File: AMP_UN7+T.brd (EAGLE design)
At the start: 31 parts

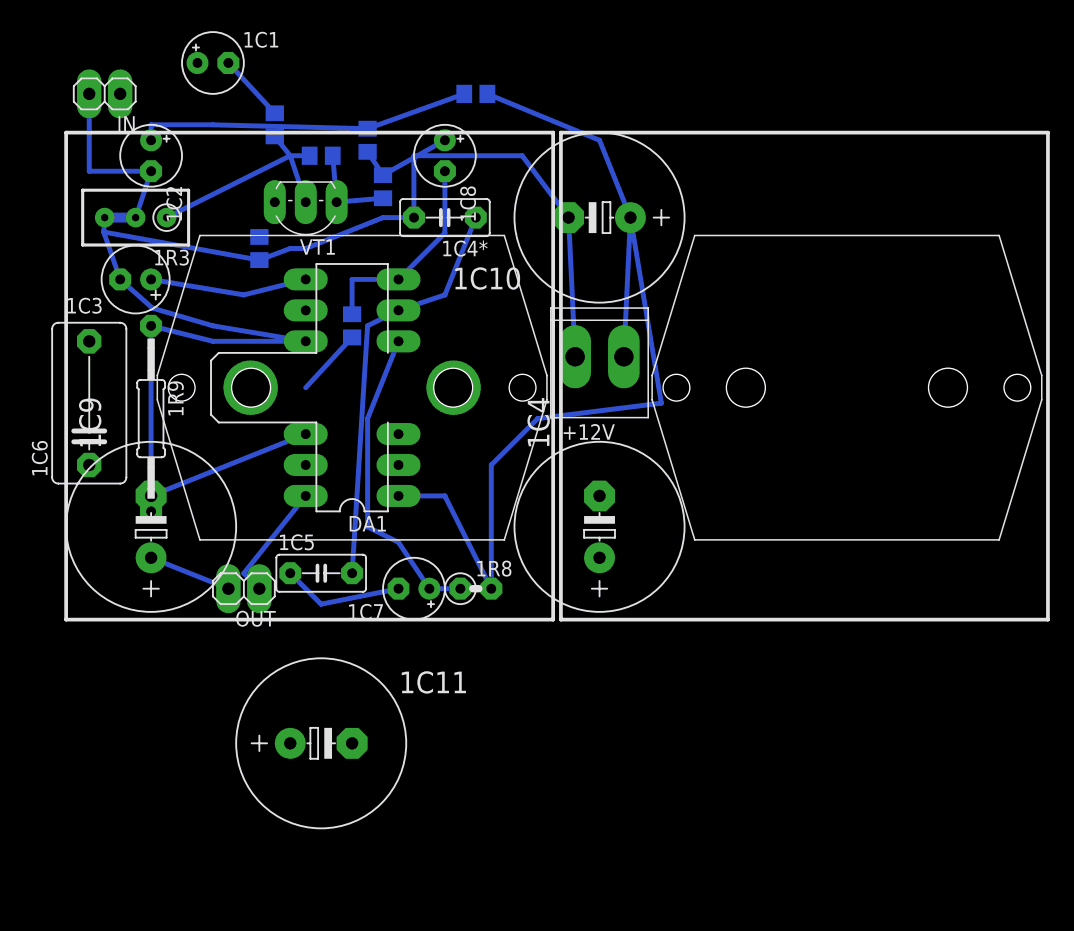
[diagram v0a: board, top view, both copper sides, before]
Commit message: 1
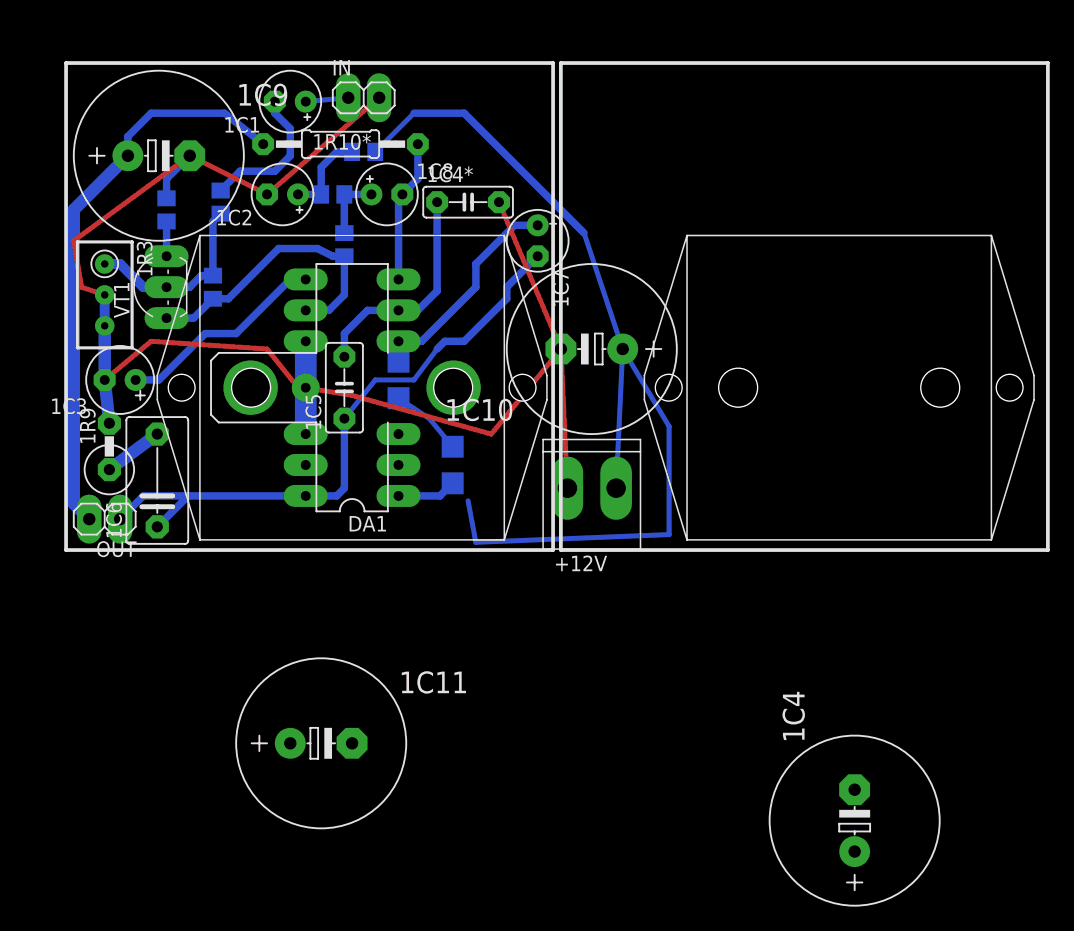
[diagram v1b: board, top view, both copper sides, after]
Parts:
- added 1R8': (no value), rcl:R1210W
- 1C4*: device rcl:C050-030X075 -> rcl:C050-025X075
- 1C6: device rcl:C102-064X133 -> rcl:C075-052X106
- 1R10*: device rcl:R0805 -> rcl:0207/12
- 1R8: device rcl:0207/2V -> rcl:R1210W
- 1R9: device rcl:0207/15 -> rcl:0411V
- moved U$1 40.4 mm to (-62.9, 84.5), turned to 0 degrees
- moved U$2 40.4 mm to (-22.2, 84.5), turned to 0 degrees
- moved 1C4 32.0 mm to (1.91, 62.2)
- moved 1C9 30.5 mm to (-55.2, 116.8), turned to 0 degrees
- moved 1C7 30.3 mm to (-24.1, 109.9), turned to 270 degrees
- moved IN 21.3 mm to (-38.4, 121.6), turned to 0 degrees
- moved 1C5 15.4 mm to (-40.0, 97.8), turned to 90 degrees
- moved 1R10* 15.0 mm to (-40.3, 117.8), flipped to the top, turned to 180 degrees
- moved 1R2 14.0 mm to (-50.8, 106.0), turned to 270 degrees
- moved VT1 13.9 mm to (-55.9, 106.0), turned to 90 degrees
- moved OUT 12.8 mm to (-59.7, 87.0)
- moved 1C2 11.3 mm to (-45.1, 113.7), turned to 180 degrees
- moved +12V 10.8 mm to (-19.7, 89.5)
- moved 1C10 10.8 mm to (-19.7, 101.0)
- moved 1R7 10.4 mm to (-38.4, 117.2)
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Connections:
- new net N$10: 1R8'.2, 1R8.1
- net GND: now also 1R9.2; no longer 1R9.1
- net N$12: now also 1R9.1; no longer 1R9.2
- net N$9: now also 1R8'.1; no longer 1R8.1
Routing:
- net OUT1-: track 12.5 -> 46.6 mm
- net OUT1+: track 20.0 -> 51.2 mm
- net N$6: track 27.5 -> 7.20 mm
- net N$1: track 7.65 -> 24.0 mm
- net N$11: track 34.1 -> 18.3 mm
- net GND: track 138.4 -> 127.9 mm, vias 0 -> 1
- net N$9: track 25.7 -> 18.2 mm
- net N$4: track 5.62 -> 11.9 mm
- net N$10: track 0.00 -> 6.04 mm
- net N$13: track 17.1 -> 11.8 mm
- net N$12: track 0.00 -> 4.90 mm
- net N$8: track 13.0 -> 17.4 mm
- net N$3: track 19.0 -> 15.4 mm
- net N$7: track 0.00 -> 3.51 mm
- net N$2: track 0.00 -> 2.86 mm
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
